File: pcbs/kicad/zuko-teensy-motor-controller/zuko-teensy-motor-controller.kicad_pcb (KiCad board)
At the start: 2 copper layers, 100 x 45 mm, 63 parts, among them J1 Conn_01x03, J10 Conn_01x03, J11 Conn_01x03, J12 Conn_01x03, J13 Conn_01x03, J14 Conn_01x02, J15 Conn_01x02, J16 Conn_01x02, J17 Conn_01x03, J18 Conn_01x03, J19 Conn_01x02, J2 Conn_01x03, J20 Conn_01x02, J21 Conn_01x02, J22 Conn_01x03, J23 Conn_01x03, J24 Conn_01x04, J25 Conn_01x03, J26 Conn_01x03, J27 Conn_01x04, J28 Conn_01x04, J29 Conn_01x04, J3 Conn_01x03, J30 Conn_01x04, J31 Conn_01x04, J32 Conn_01x04, J33 Conn_01x04, J4 Conn_01x02, J5 Conn_01x03, J6 Conn_01x03, J7 Conn_01x03, J8 Conn_01x03, J9 Conn_01x03, Q1 BSS138, Q2 BSS138, U1 ACS712xLCTR-20A, U2 Teensy4.0, U3 ULN2003

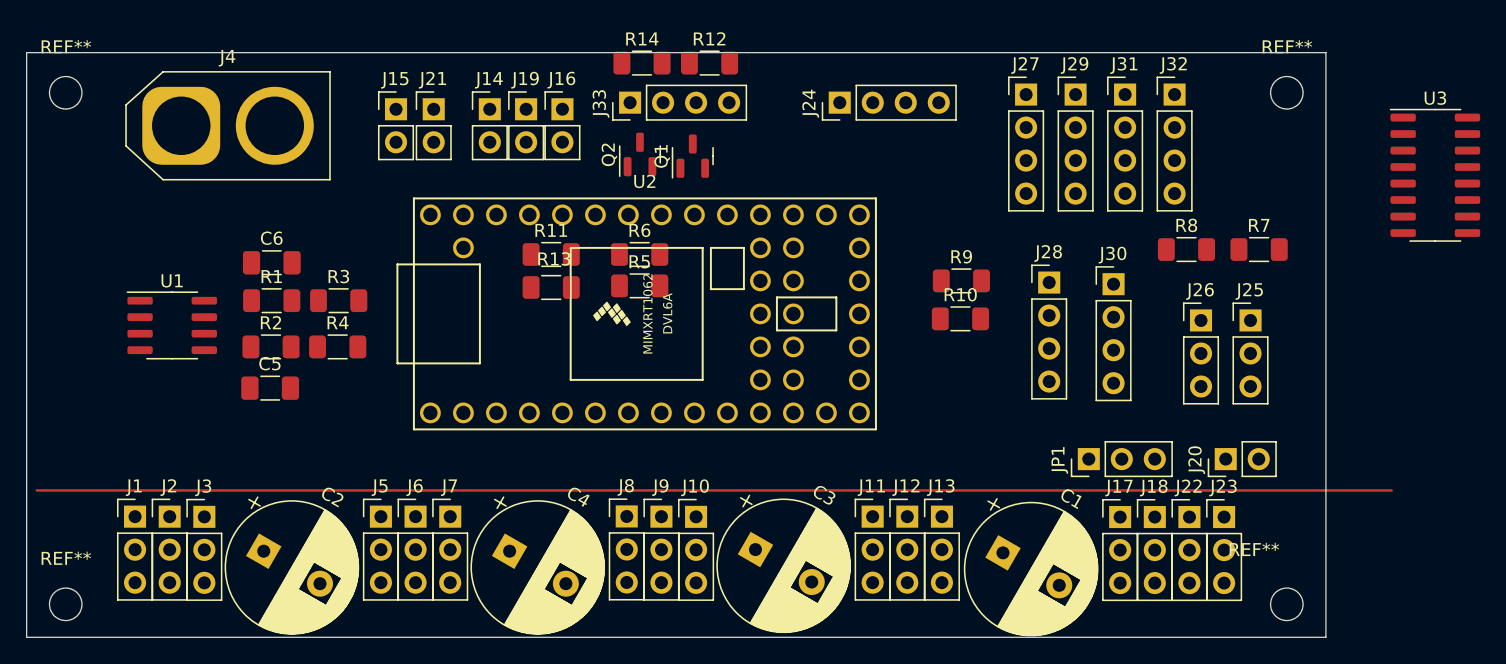
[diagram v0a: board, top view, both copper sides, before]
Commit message: pcb update
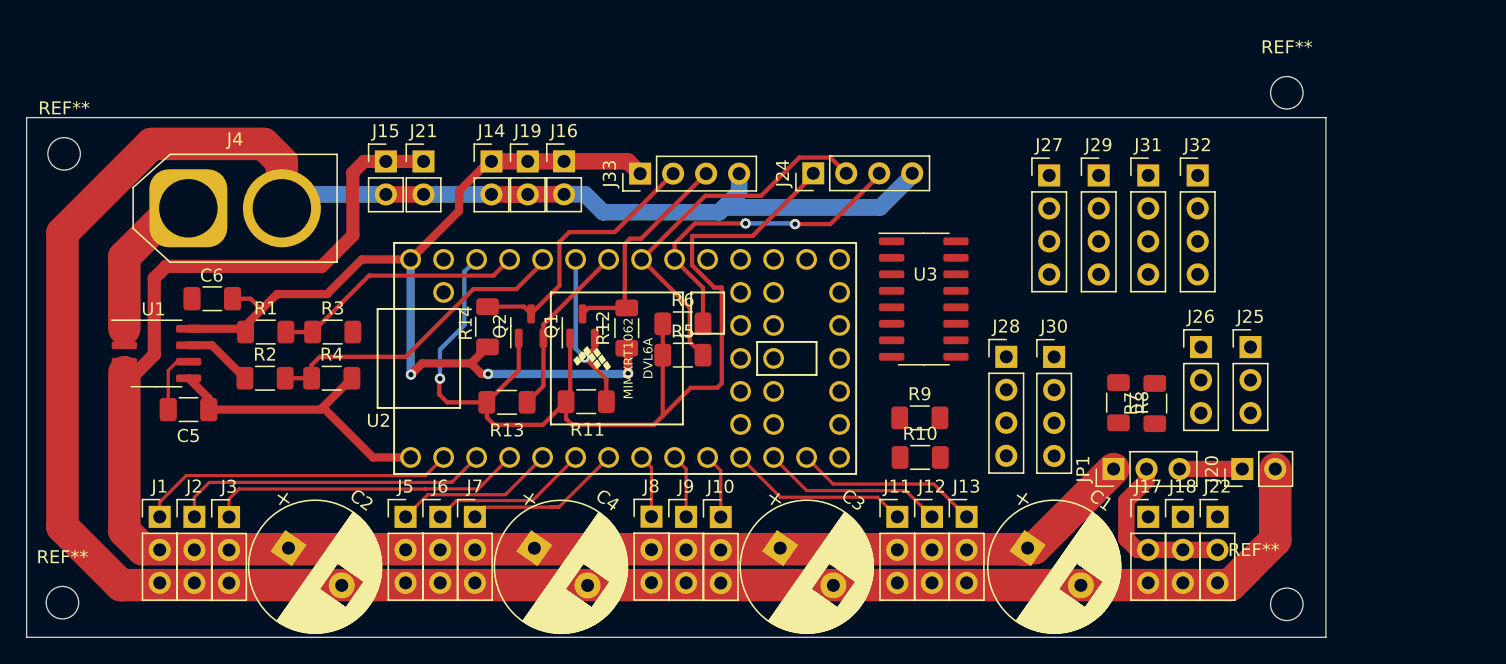
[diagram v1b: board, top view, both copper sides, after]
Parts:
- removed J23: Conn_01x03, Connector_PinHeader_2.54mm:PinHeader_1x03_P2.54mm_Vertical
- moved U3 40.5 mm to (143.5, 70.5)
- moved R14 23.5 mm to (109.9, 72.6), turned to 90 degrees
- moved R12 21.4 mm to (120.7, 72.7), turned to 90 degrees
- moved Q2 15.6 mm to (113.3, 72.6)
- moved Q1 15.6 mm to (117.2, 72.6)
- moved R7 14.3 mm to (161.3, 78.5), turned to 90 degrees
- moved R8 12.9 mm to (158.5, 78.5), turned to -90 degrees
- moved R11 11.6 mm to (117.5, 78.4)
- moved R10 11.1 mm to (143.2, 82.7)
- moved R9 11.0 mm to (143.2, 79.6)
- moved R13 9.47 mm to (111.4, 78.4)
- moved J30 7.23 mm to (153.5, 74.9)
- moved J28 6.60 mm to (149.9, 74.9)
- moved C5 6.50 mm to (86.9, 79.0)
- moved J27 6.47 mm to (153.2, 61.0)
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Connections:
- J17 pad 1: Net-(J17-Pad1) -> AUX_M1
- J17 pad 2: AUX_M1 -> Net-(J18-Pad2)
- J18 pad 1: Net-(J17-Pad1) -> AUX_M2
- J18 pad 2: AUX_M2 -> Net-(J18-Pad2)
- J22 pad 1: Net-(J17-Pad1) -> AUX_M3
- J22 pad 2: AUX_M3 -> Net-(J18-Pad2)
- JP1 pad 2: Net-(J17-Pad1) -> Net-(J18-Pad2)
- U2 pad 14: unconnected-(U2-Pad14) -> AUX_M1
- U2 pad 21: unconnected-(U2-Pad21) -> OUT4
- U2 pad 22: unconnected-(U2-Pad22) -> OUT3
- U2 pad 23: unconnected-(U2-Pad23) -> OUT2
- U2 pad 24: unconnected-(U2-Pad24) -> OUT1
- U2 pad 29: unconnected-(U2-Pad29) -> CSENSE
- U2 pad 30: unconnected-(U2-Pad30) -> VSENSE
- U2 pad 35: unconnected-(U2-Pad35) -> SDL1
- U2 pad 36: unconnected-(U2-Pad36) -> SDA1
- U2 pad 37: unconnected-(U2-Pad37) -> NEO2
- U2 pad 38: unconnected-(U2-Pad38) -> NEO1
- U2 pad 39: unconnected-(U2-Pad39) -> SW1
- U2 pad 40: unconnected-(U2-Pad40) -> AUX_M3
- U2 pad 41: unconnected-(U2-Pad41) -> SW3
- U2 pad 42: unconnected-(U2-Pad42) -> SW2
- U2 pad 43: unconnected-(U2-Pad43) -> SW4
- U2 pad 44: unconnected-(U2-Pad44) -> AUX_M2
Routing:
- net GND: track 0.00 -> 229.4 mm
- net +BATT: track 0.00 -> 127.3 mm
- net +3V3: track 0.00 -> 80.6 mm, vias 0 -> 1
- net +5V: track 0.00 -> 74.4 mm, vias 0 -> 3
- net SCL0: track 0.00 -> 28.8 mm
- net M2: track 0.00 -> 25.3 mm
- net SDA0: track 0.00 -> 25.2 mm, vias 0 -> 2
- net M1: track 0.00 -> 24.4 mm
- net CSENSE: track 0.00 -> 24.3 mm
- net M3: track 0.00 -> 24.3 mm
- net Net-(J33-Pad2): track 0.00 -> 21.0 mm
- net VSENSE: track 0.00 -> 19.5 mm
- net Net-(J33-Pad3): track 0.00 -> 17.1 mm
- net M12: track 0.00 -> 14.4 mm
- net M11: track 0.00 -> 14.1 mm
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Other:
- board size 100 x 45 mm -> 100 x 40 mm
